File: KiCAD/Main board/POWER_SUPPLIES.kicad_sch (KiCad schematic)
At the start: 32 parts, among them U18 12V, U19 5V, U20 8V, U21 15V, U23 LIN_REG_±5V, U24 LIN_REG_±12V, U28 12V, U29 AP2111H-3.3TRG1, U31 AP2111H-3.3TRG1, U9 SEPIC_-15V_LT3579

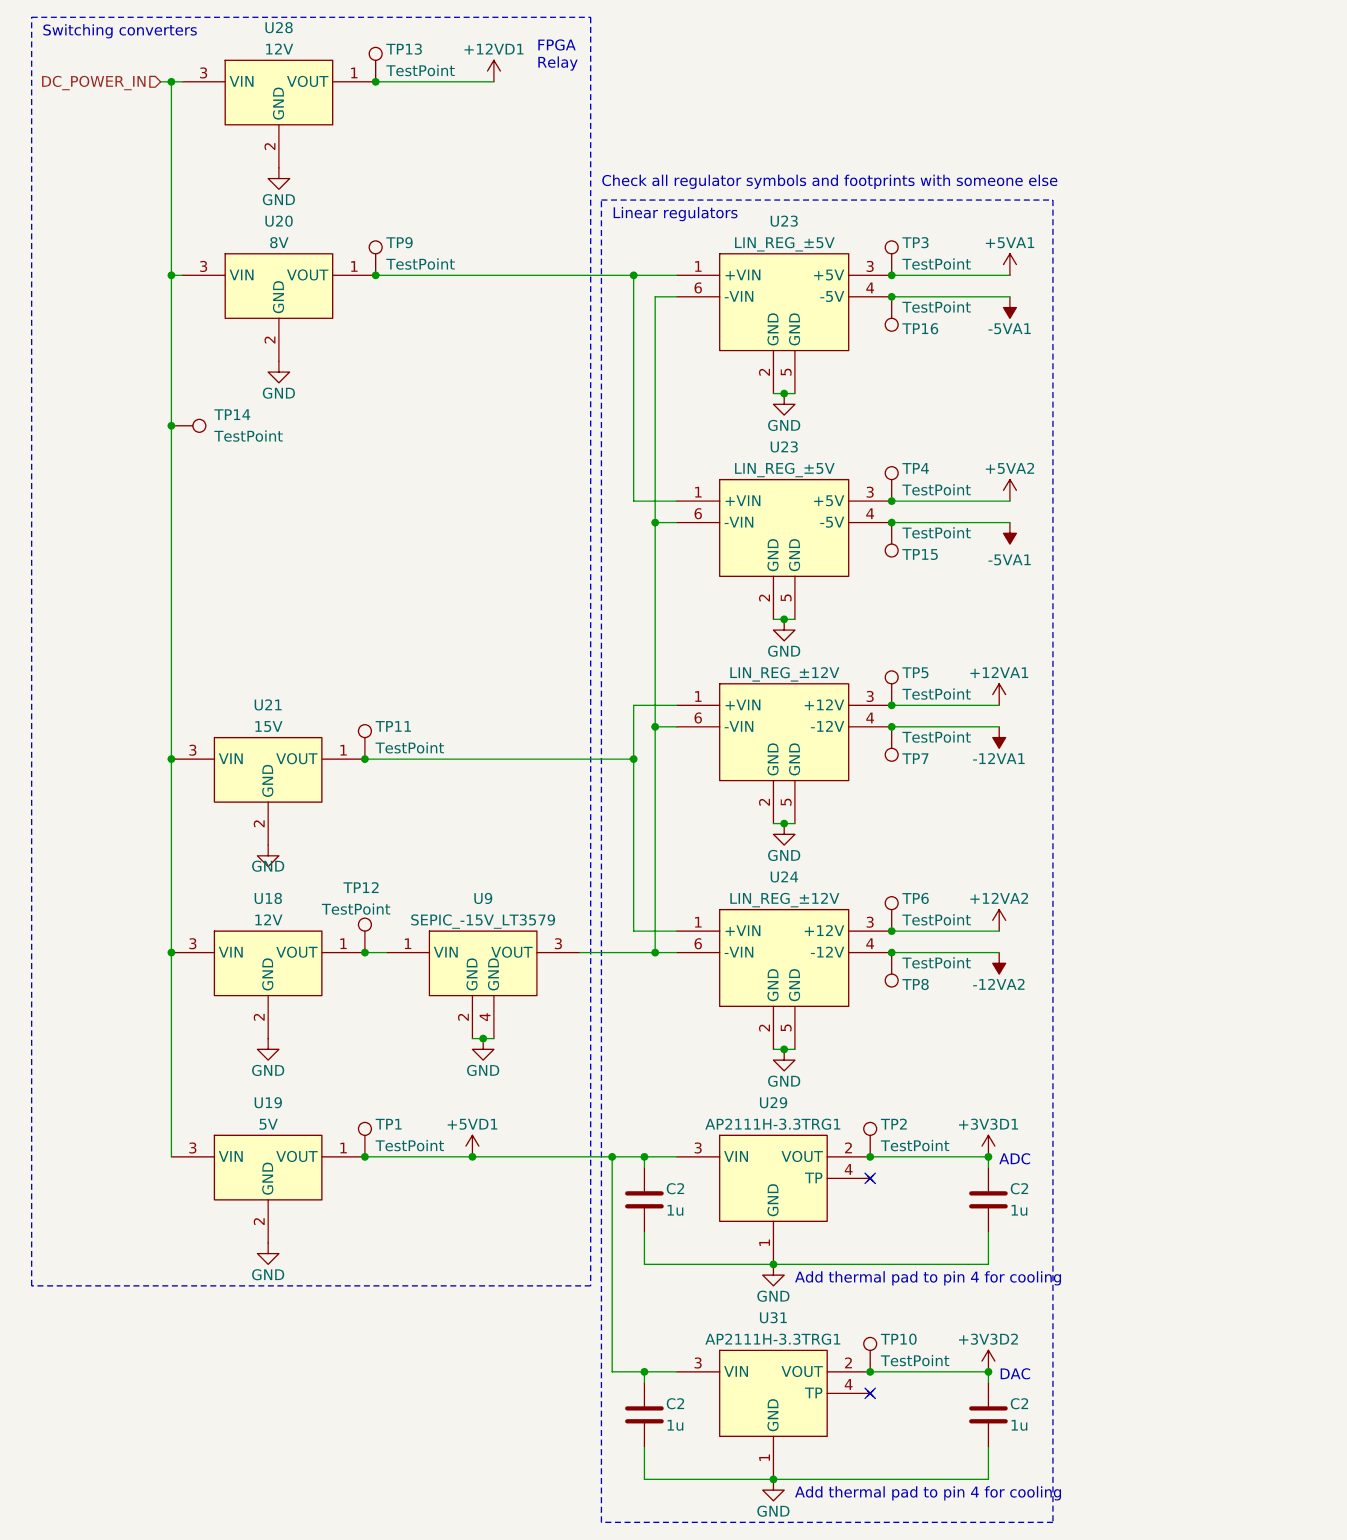
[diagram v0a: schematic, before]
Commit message: Main board
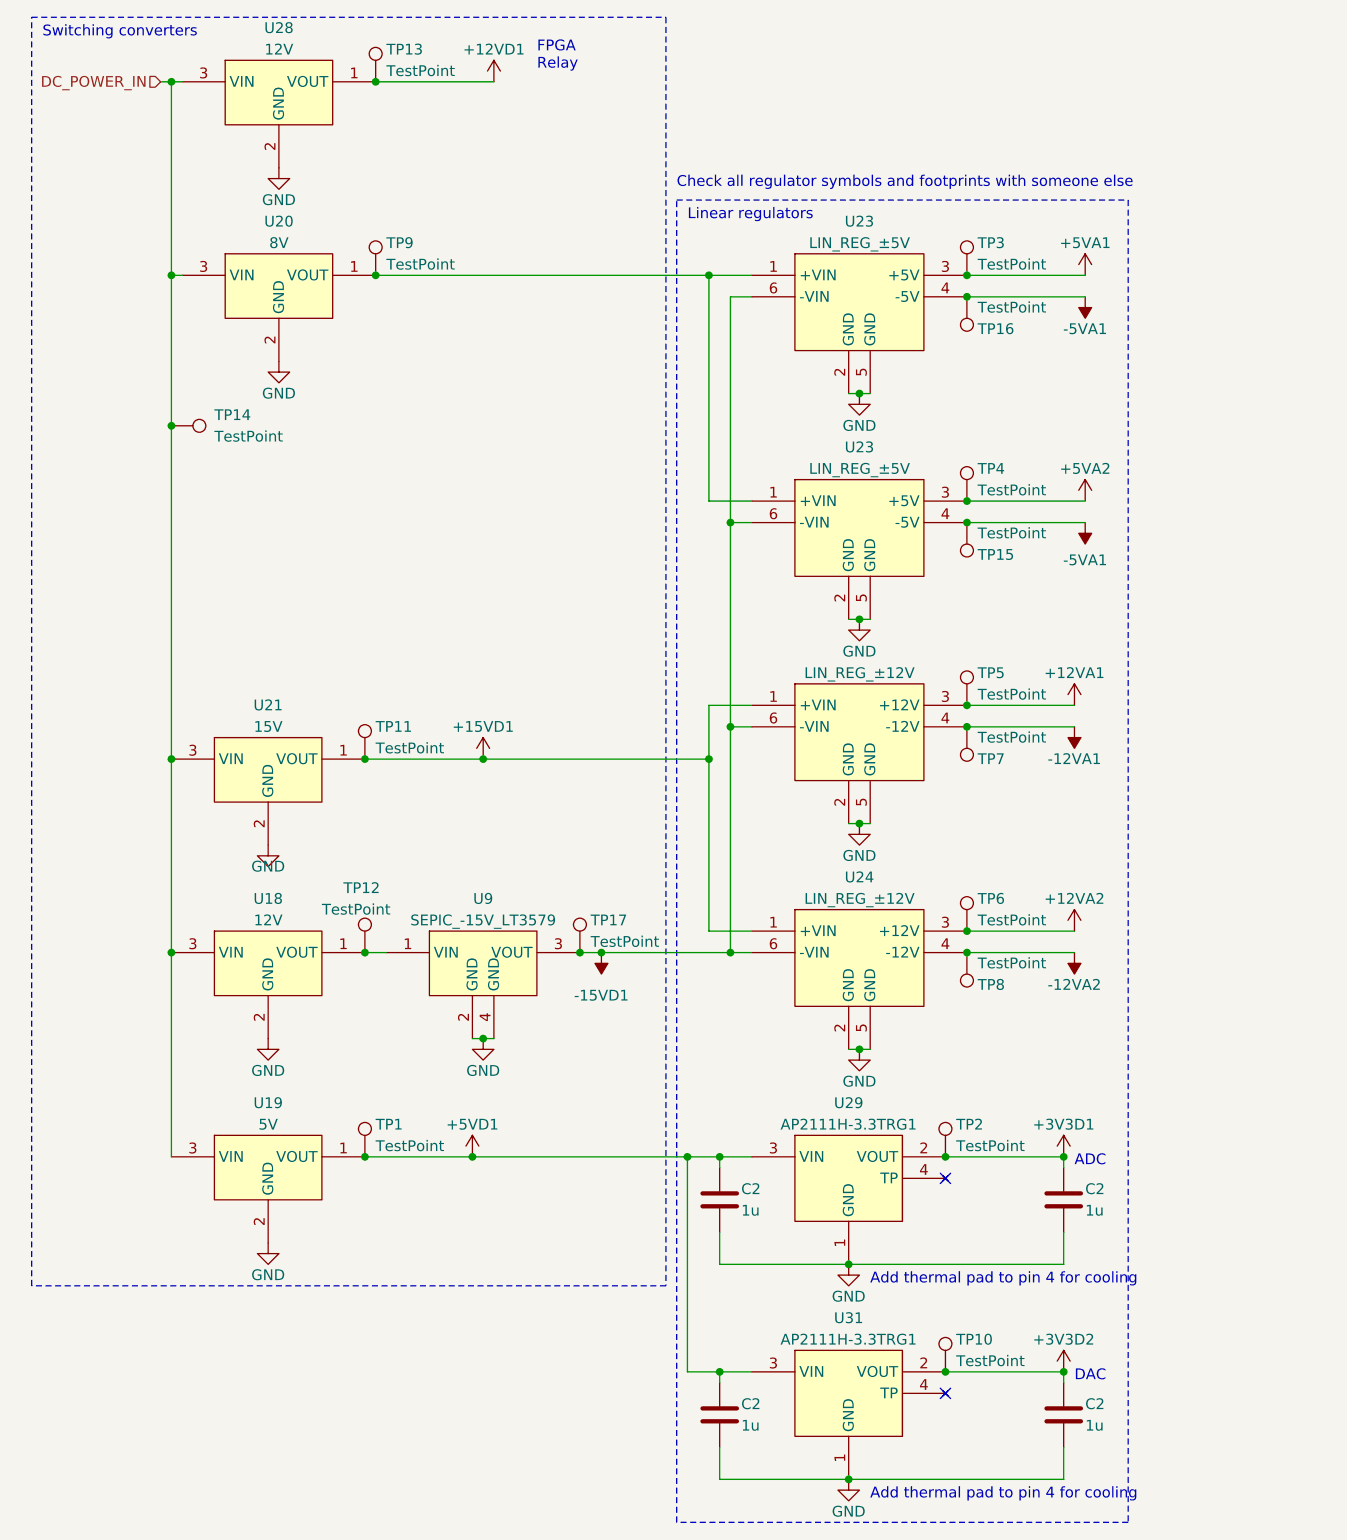
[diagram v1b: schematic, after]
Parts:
- added TP17: TestPoint, TestPoint:TestPoint_Pad_D2.0mm, symbol Connector:TestPoint
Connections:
- net -15VD1: now reaches U23.6 (-VIN), U23.6 (-VIN), U24.6 (-VIN), U24.6 (-VIN), U9.3 (VOUT)
- net -15VD1: now also TP17.1
- net +15VD1: now reaches TP11.1, U21.1 (VOUT), U24.1 (+VIN), U24.1 (+VIN)
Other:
- moved on the sheet: C2, TP10, TP15, TP16, TP2, TP3, TP4, TP5, TP6, TP7, TP8, U23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

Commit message: Worked on main board schematic
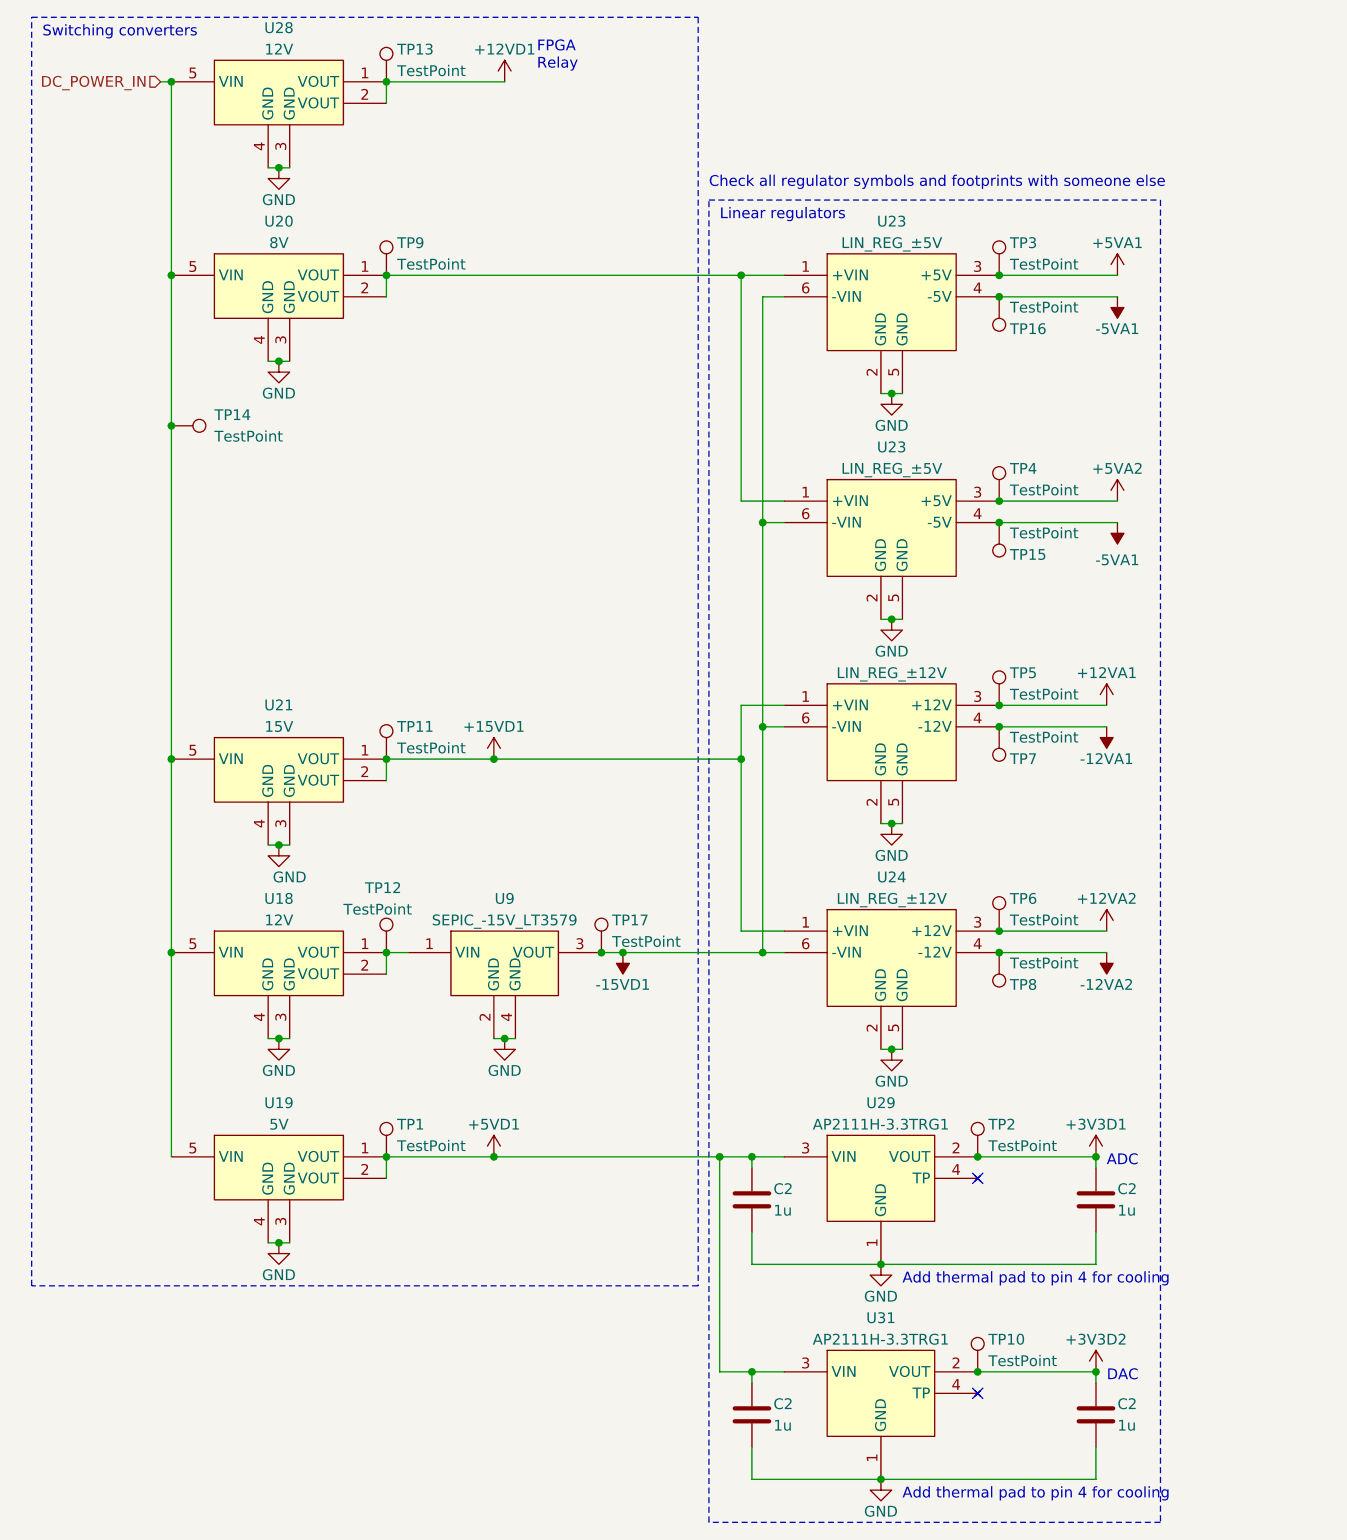
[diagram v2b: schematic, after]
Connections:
- net +12VD1: now also U28.2 (VOUT)
- net +15VD1: now also U21.2 (VOUT)
- net +5VD1: now also U19.2 (VOUT)
- net DC_POWER_IN: now also U18.5 (VIN), U19.5 (VIN), U20.5 (VIN), U21.5 (VIN), U28.5 (VIN); no longer U18.3 (VIN), U19.3 (VIN), U20.3 (VIN), U21.3 (VIN), U28.3 (VIN)
- net GND: now also U18.3 (GND), U18.4 (GND), U19.3 (GND), U19.4 (GND), U20.3 (GND), U20.4 (GND), U21.3 (GND), U21.4 (GND), U28.3 (GND), U28.4 (GND); no longer U18.2 (GND), U19.2 (GND), U20.2 (GND), U21.2 (GND), U28.2 (GND)
- net at TP9.1, U20.1 (VOUT), U23.1 (+VIN)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: now also U20.2 (VOUT)
- net at TP12.1, U18.1 (VOUT), U9.1 (VIN): now also U18.2 (VOUT)
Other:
- moved on the sheet: C2, TP1, TP10, TP11, TP12, TP13, TP15, TP16, TP17, TP2, TP3, TP4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
